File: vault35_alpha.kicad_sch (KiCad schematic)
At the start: 131 parts, among them J1 AVR-ISP-6, SW1 SW_PUSH, SW2 RotaryEncoder_Switch, SW3 RotaryEncoder_Switch, SW4 RotaryEncoder_Switch, SW5 SW_PUSH, SW6 SW_PUSH, U1 SRV05-4, U2 ATmega32U4-M, X1 Crystal_GND24_Small

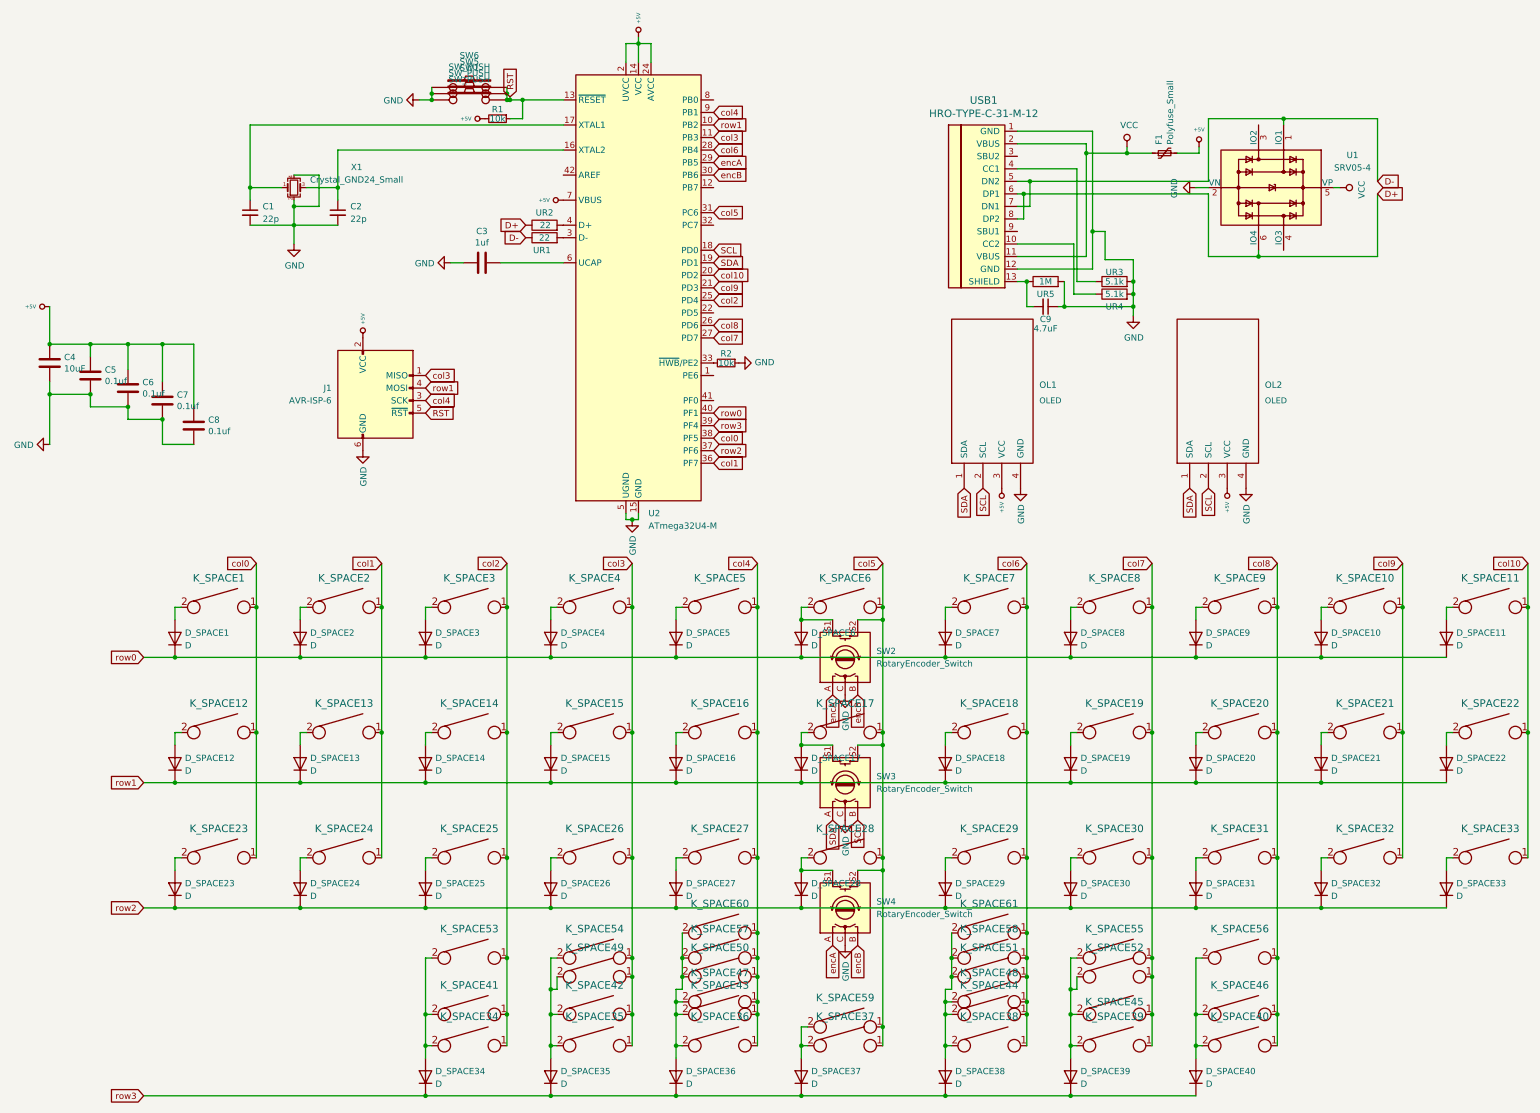
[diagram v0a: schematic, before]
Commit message: Update
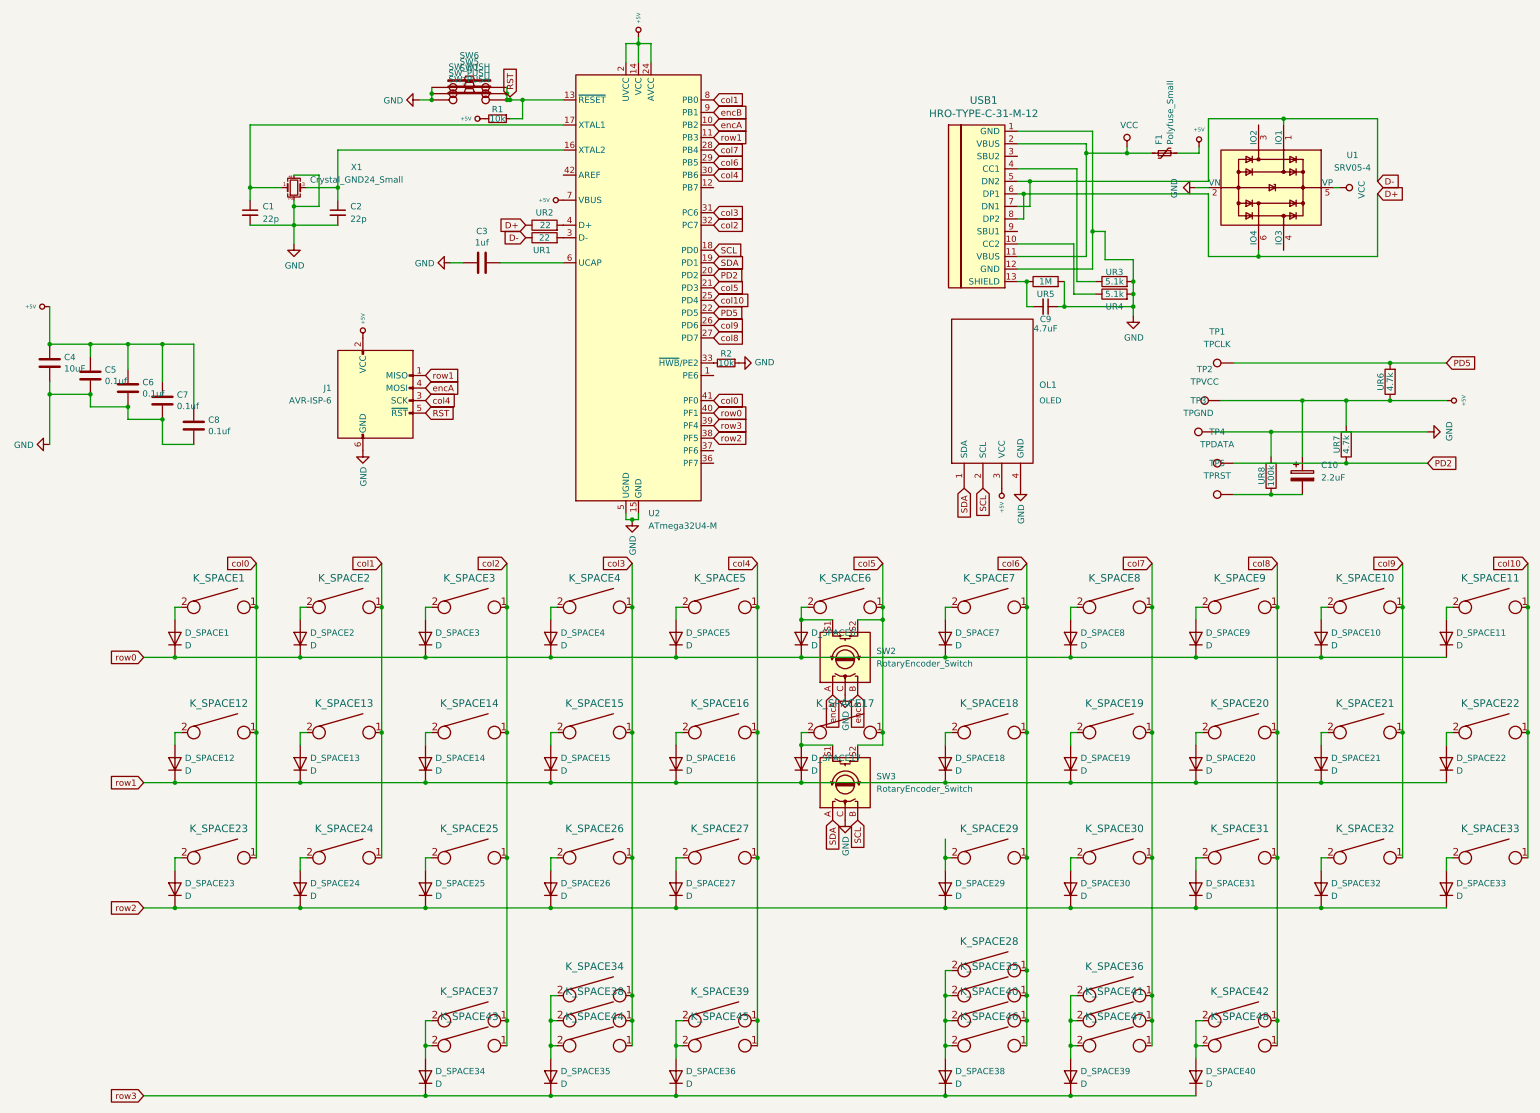
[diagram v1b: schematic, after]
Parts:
- removed D_SPACE28, D_SPACE37: D, Diode_SMD:D_SOD-123, symbol Device:D
- removed K_SPACE49, K_SPACE52, K_SPACE53, K_SPACE54, K_SPACE55, K_SPACE56: KEYSW, MX_Only:MXOnly-1.25U-NoLED, symbol keyboard_parts:KEYSW
- removed K_SPACE50, K_SPACE51: KEYSW, MX_Only:MXOnly-1.75U-NoLED, symbol keyboard_parts:KEYSW
- removed K_SPACE57, K_SPACE58, K_SPACE59: KEYSW, MX_Only:MXOnly-3U-ReversedStabilizers-NoLED, symbol keyboard_parts:KEYSW
- removed K_SPACE60, K_SPACE61: KEYSW, MX_Only:MXOnly-1.5U-NoLED, symbol keyboard_parts:KEYSW
- removed OL2: OLED, kbd:OLED_v2, symbol kbd:OLED
- removed SW4: RotaryEncoder_Switch, encoder:RotaryEncoder_Alps_EC11E-Switch_Vertical_H20mm, symbol Device:RotaryEncoder_Switch
- added C10: 2.2uF, Capacitor_SMD:C_0805_2012Metric_Pad1.18x1.45mm_HandSolder, symbol Device:C_Polarized
- added TP1: TPCLK, TestPoint:TestPoint_THTPad_1.0x1.0mm_Drill0.5mm, symbol Connector:TestPoint
- added TP2: TPVCC, TestPoint:TestPoint_THTPad_1.0x1.0mm_Drill0.5mm, symbol Connector:TestPoint
- added TP3: TPGND, TestPoint:TestPoint_THTPad_1.0x1.0mm_Drill0.5mm, symbol Connector:TestPoint
- added TP4: TPDATA, TestPoint:TestPoint_THTPad_1.0x1.0mm_Drill0.5mm, symbol Connector:TestPoint
- added TP5: TPRST, TestPoint:TestPoint_THTPad_1.0x1.0mm_Drill0.5mm, symbol Connector:TestPoint
- added UR6, UR7: 4.7k, Resistor_SMD:R_0805_2012Metric_Pad1.20x1.40mm_HandSolder, symbol device:R
- added UR8: 100k, Resistor_SMD:R_0805_2012Metric_Pad1.20x1.40mm_HandSolder, symbol device:R
- K_SPACE23, K_SPACE28, K_SPACE33, K_SPACE39: footprint MX_Only:MXOnly-1U-NoLED -> MX_Only:MXOnly-1.5U-NoLED
- K_SPACE34: footprint MX_Only:MXOnly-1.5U-NoLED -> MX_Only:MXOnly-1.25U-NoLED
- K_SPACE35, K_SPACE45: footprint MX_Only:MXOnly-1U-NoLED -> MX_Only:MXOnly-1.75U-NoLED
- K_SPACE36, K_SPACE37, K_SPACE38, K_SPACE41, K_SPACE42: footprint MX_Only:MXOnly-1U-NoLED -> MX_Only:MXOnly-1.25U-NoLED
- K_SPACE40: footprint MX_Only:MXOnly-1.5U-NoLED -> MX_Only:MXOnly-3U-ReversedStabilizers-NoSwitch
- K_SPACE43, K_SPACE44: footprint MX_Only:MXOnly-2U-ReversedStabilizers-NoLED -> MX_Only:MXOnly-1U-NoLED
- K_SPACE46: footprint MX_Only:MXOnly-1U-NoLED -> MX_Only:MXOnly-6U-Centered-ReversedStabilizers-NoLED
- K_SPACE47: footprint MX_Only:MXOnly-2.25U-ReversedStabilizers-NoLED -> MX_Only:MXOnly-1U-NoLED
- K_SPACE48: footprint MX_Only:MXOnly-2.75U-ReversedStabilizers-NoLED -> MX_Only:MXOnly-1U-NoLED
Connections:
- net +5V: now also C10.1, TP2.1, UR6.1, UR7.2
- net GND: now also TP3.1, UR8.2
- net col0: now also U2.41 (PF0); no longer U2.38 (PF5)
- net col1: now also U2.8 (PB0); no longer U2.36 (PF7)
- net col10: now also U2.25 (PD4); no longer U2.20 (PD2)
- net col2: now also K_SPACE37.1, K_SPACE43.1, U2.32 (PC7); no longer K_SPACE34.1, K_SPACE41.1, U2.25 (PD4)
- net col3: now also K_SPACE34.1, K_SPACE38.1, K_SPACE44.1, U2.31 (PC6); no longer J1.1 (MISO), K_SPACE35.1, K_SPACE42.1, U2.11 (PB3)
- net col4: now also K_SPACE39.1, K_SPACE45.1, U2.30 (PB6); no longer K_SPACE36.1, K_SPACE43.1, K_SPACE47.1, U2.9 (PB1)
- net col5: now also U2.21 (PD3); no longer K_SPACE28.1, K_SPACE37.1, U2.31 (PC6)
- net col6: now also K_SPACE28.1, K_SPACE35.1, K_SPACE40.1, K_SPACE46.1, U2.29 (PB5); no longer K_SPACE38.1, K_SPACE44.1, K_SPACE48.1, U2.28 (PB4)
- net col7: now also K_SPACE36.1, K_SPACE41.1, K_SPACE47.1, U2.28 (PB4); no longer K_SPACE39.1, K_SPACE45.1, U2.27 (PD7)
- net col8: now also K_SPACE42.1, K_SPACE48.1, U2.27 (PD7); no longer K_SPACE40.1, K_SPACE46.1, U2.26 (PD6)
- net col9: now also U2.26 (PD6); no longer U2.21 (PD3)
- net encA: now also J1.4 (MOSI), U2.10 (PB2); no longer U2.29 (PB5)
- net encB: now also U2.9 (PB1); no longer U2.30 (PB6)
- net row1: now also J1.1 (MISO), U2.11 (PB3); no longer J1.4 (MOSI), U2.10 (PB2)
- net row2: now also U2.38 (PF5); no longer U2.37 (PF6)
- net at K_SPACE38.2, K_SPACE44.2: now also D_SPACE35.2 (A), K_SPACE34.2; no longer D_SPACE38.2 (A), K_SPACE48.2
- net at K_SPACE28.2: now also D_SPACE38.2 (A), K_SPACE35.2, K_SPACE40.2, K_SPACE46.2
- net at K_SPACE37.2: now also D_SPACE34.2 (A), K_SPACE43.2
- net at K_SPACE36.2, K_SPACE47.2: now also D_SPACE39.2 (A), K_SPACE41.2; no longer D_SPACE36.2 (A), K_SPACE43.2
- net PD5: now reaches U2.22 (PD5)
- net PD5: now also TP1.1, UR6.2
- net at K_SPACE39.2, K_SPACE45.2: now also D_SPACE36.2 (A); no longer D_SPACE39.2 (A)
- new net: D_SPACE40.2 (A), K_SPACE42.2, K_SPACE48.2
- new net: C10.2, TP5.1, UR8.1
- new net PD2: TP4.1, U2.20 (PD2), UR7.1

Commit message: update with TP, alpha stagger
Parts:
- U2: footprint Package_DFN_QFN:QFN-44-1EP_7x7mm_P0.5mm_EP5.2x5.2mm -> Package_DFN_QFN:QFN-44-1EP_7x7mm_P0.5mm_EP5.2x5.2mm_ThermalVias
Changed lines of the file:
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@@
       (effects (font (size 1.27 1.27)) (justify left))
     )
-    (property "Footprint" "Package_DFN_QFN:QFN-44-1EP_7x7mm_P0.5mm_EP5.2x5.2mm" (id 2) (at 156.21 73.66 0)
+    (property "Footprint" "Package_DFN_QFN:QFN-44-1EP_7x7mm_P0.5mm_EP5.2x5.2mm_ThermalVias" (id 2) (at 156.21 73.66 0)
       (effects (font (size 1.27 1.27) italic) hide)
     )
@@
     )
     (path "/41996209-b9ca-4c2f-9bac-165f421bc575"
-      (reference "U2") (unit 1) (value "ATmega32U4-M") (footprint "Package_DFN_QFN:QFN-44-1EP_7x7mm_P0.5mm_EP5.2x5.2mm")
+      (reference "U2") (unit 1) (value "ATmega32U4-M") (footprint "Package_DFN_QFN:QFN-44-1EP_7x7mm_P0.5mm_EP5.2x5.2mm_ThermalVias")
     )
     (path "/585f9e9f-dfe7-4dd8-8c55-e7e89ca5db61"
